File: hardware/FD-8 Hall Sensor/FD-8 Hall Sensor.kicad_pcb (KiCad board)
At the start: 2 copper layers, 27.9 x 45.7 mm, 19 parts, among them J1 Panel connections, J2 ICSP Programming, J3 Hall sensor input, J4 Extra GPIO, U1 LM2940T-5.0_NOPB, U2 ATtiny13A-P, U3 MCP42010

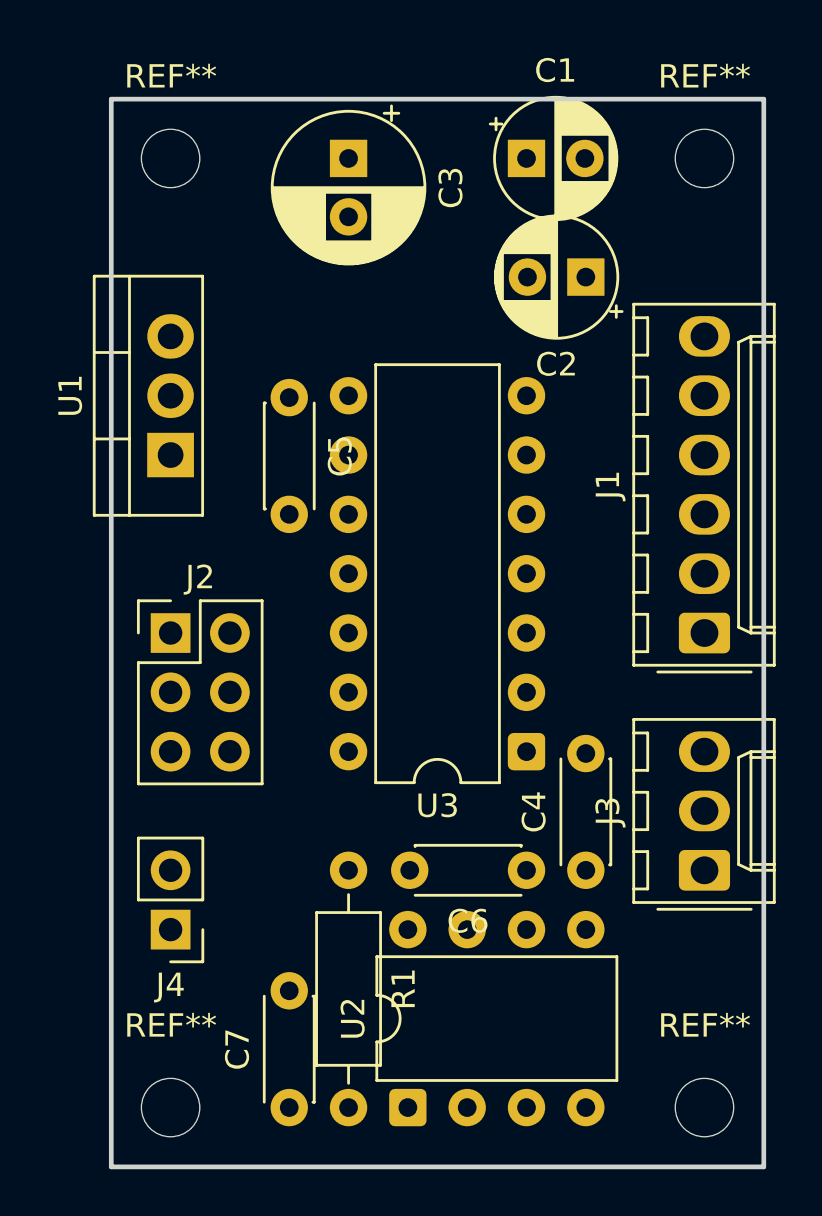
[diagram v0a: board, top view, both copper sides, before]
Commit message: routing etc.
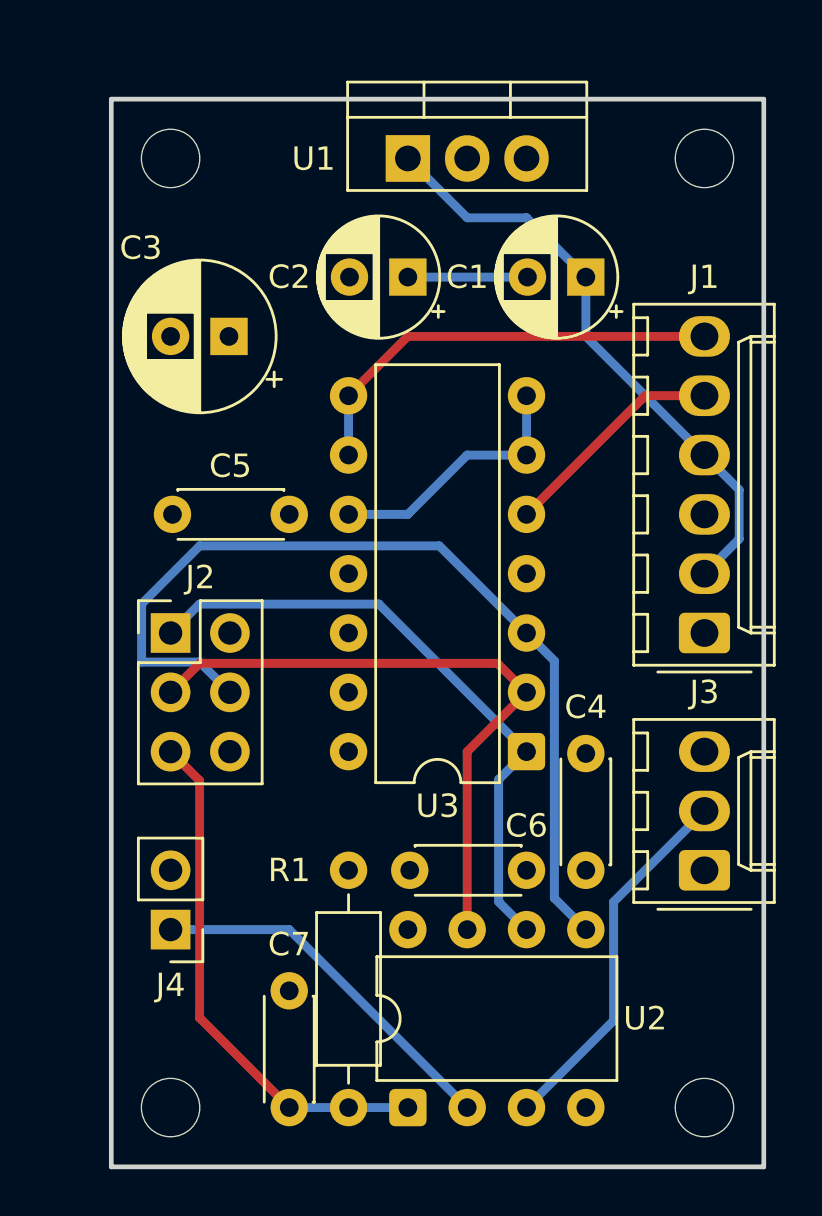
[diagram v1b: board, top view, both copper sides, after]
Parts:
- moved U1 16.3 mm to (188.0, 76.2), turned to 0 degrees
- moved C3 9.18 mm to (180.3, 83.8), turned to 180 degrees
- moved C2 7.62 mm to (188.0, 81.3)
- moved C1 5.68 mm to (195.6, 81.3), turned to 180 degrees
- moved C5 5.00 mm to (182.9, 91.4), turned to 180 degrees
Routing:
- net /ICSP_MOSI: track 0.00 -> 39.6 mm
- net /ICSP_SCK: track 0.00 -> 27.5 mm
- net /ICSP_MISO: track 0.00 -> 27.0 mm
- net Net-(J1-Pin_2): track 0.00 -> 25.8 mm
- net /RESET: track 0.00 -> 22.4 mm
- net /PEDAL_TIP: track 0.00 -> 18.8 mm
- net Net-(J3-Pin_2): track 0.00 -> 15.9 mm
- net Net-(J4-Pin_1): track 0.00 -> 15.9 mm
- net Net-(U3-PA1): track 0.00 -> 11.2 mm
- net /PEDAL_SLEEVE: track 0.00 -> 9.72 mm
- net Net-(C1-Pad2): track 0.00 -> 5.12 mm
- added copper zone on In2.Cu, net +5V
- added copper zone on In1.Cu, net GND
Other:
- copper layers 2 -> 4
